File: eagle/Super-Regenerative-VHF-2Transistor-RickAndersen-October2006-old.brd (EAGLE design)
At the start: 25 parts, among them SW1 SL-SW-1P-2T-H, T1 2N3904, T2 2N3904

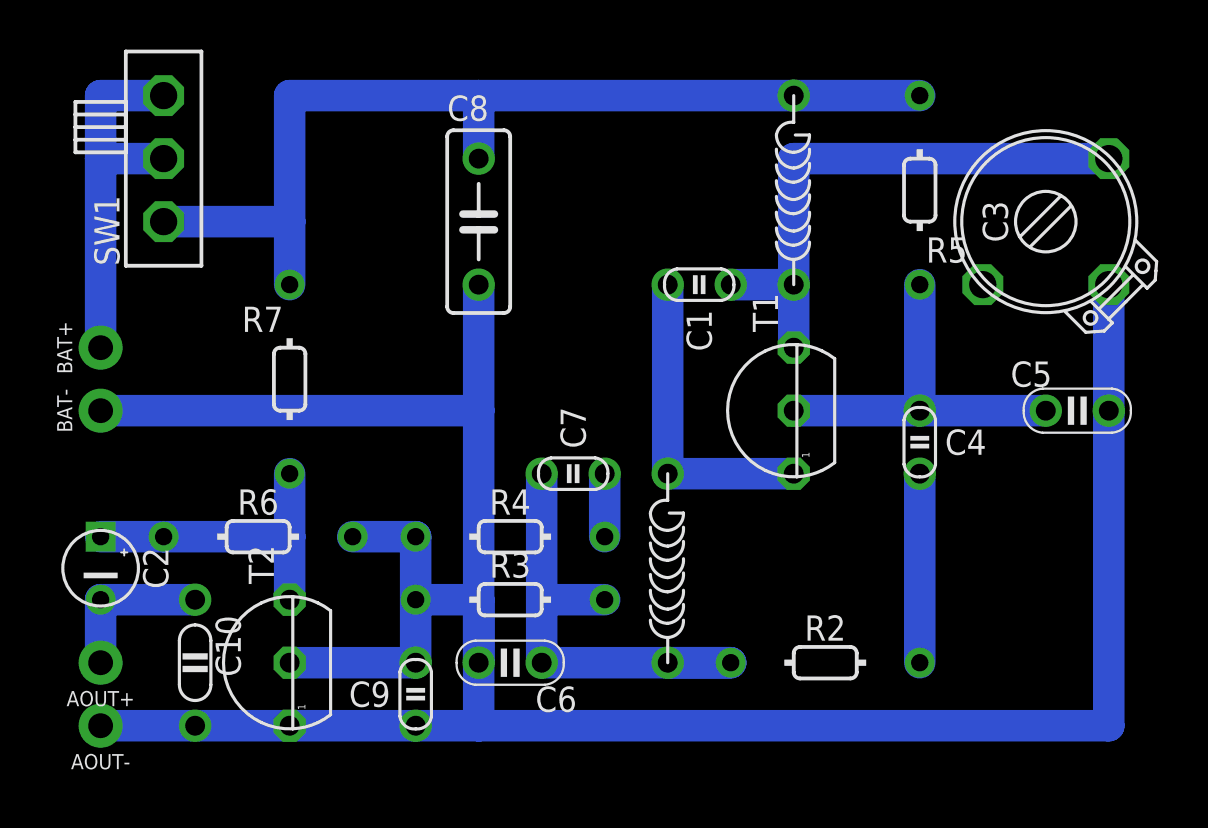
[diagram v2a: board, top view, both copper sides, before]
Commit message: updated libraries
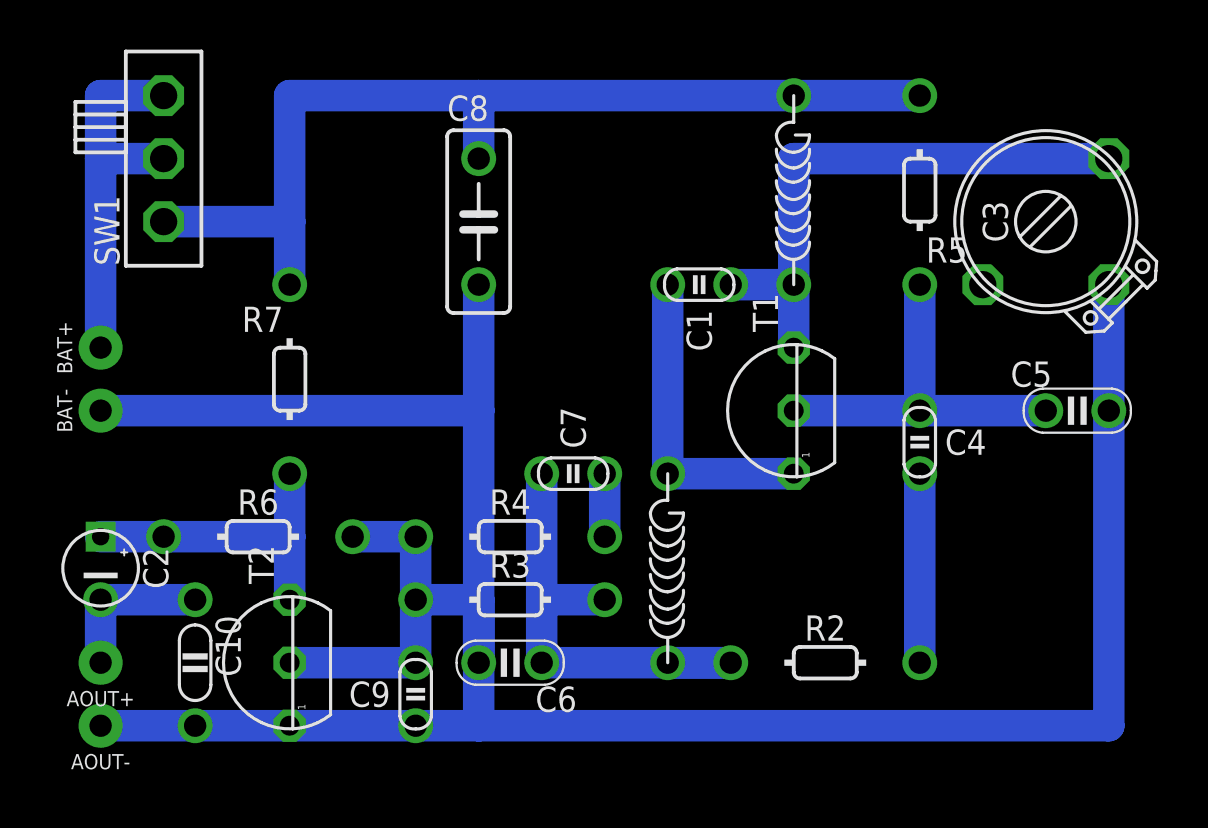
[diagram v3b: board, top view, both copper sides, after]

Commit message: ...
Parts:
- R2: value 12k -> 12kΩ
- R3: value 10k -> 10kΩ
- R4: value 22k -> 22kΩ
- R5: value 330k -> 330kΩ
- R6: value 220k -> 220kΩ
- R7: value 4.7k -> 4.7kΩ
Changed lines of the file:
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@@
 <element name="L1" library="r" package="L-02/7V" value="6turns on d=0.7mm" x="30.48" y="24.13" rot="R180"/>
 <element name="L2" library="r" package="L-02/7V" value="6 turns #22 on BIC pen" x="25.4" y="8.89" rot="R180"/>
-<element name="R2" library="r" package="0202/7" value="12k" x="31.75" y="5.08" rot="R270"/>
-<element name="R3" library="r" package="0202/7" value="10k" x="19.05" y="7.62" rot="R270"/>
-<element name="R4" library="r" package="0202/7" value="22k" x="19.05" y="10.16" rot="R270"/>
-<element name="R5" library="r" package="0202/7-V" value="330k" x="35.56" y="24.13" rot="R180"/>
+<element name="R2" library="r" package="0202/7" value="12kΩ" x="31.75" y="5.08" rot="R270"/>
+<element name="R3" library="r" package="0202/7" value="10kΩ" x="19.05" y="7.62" rot="R270"/>
+<element name="R4" library="r" package="0202/7" value="22kΩ" x="19.05" y="10.16" rot="R270"/>
+<element name="R5" library="r" package="0202/7-V" value="330kΩ" x="35.56" y="24.13" rot="R180"/>
 <element name="SW1" library="sw" package="SLSW-1P2T-H" value="SL-SW-1P-2T-H" x="5.08" y="25.4" rot="R90"/>
 <element name="C9" library="c" package="C025-015X024" value="10n" x="15.24" y="3.81"/>
-<element name="R6" library="r" package="0202/7" value="220k" x="8.89" y="10.16" rot="R270"/>
-<element name="R7" library="r" package="0202/7-V" value="4.7k" x="10.16" y="16.51"/>
+<element name="R6" library="r" package="0202/7" value="220kΩ" x="8.89" y="10.16" rot="R270"/>
+<element name="R7" library="r" package="0202/7-V" value="4.7kΩ" x="10.16" y="16.51"/>
 <element name="C2" library="c" package="E2,5-3" value="2.2u" x="2.54" y="8.89"/>
 <element name="C10" library="c" package="C050-020X036" value="47n" x="6.35" y="5.08" rot="R270"/>
